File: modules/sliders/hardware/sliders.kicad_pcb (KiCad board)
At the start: 2 copper layers, 157.5 x 96.5 mm, 10 parts, among them J5 Button

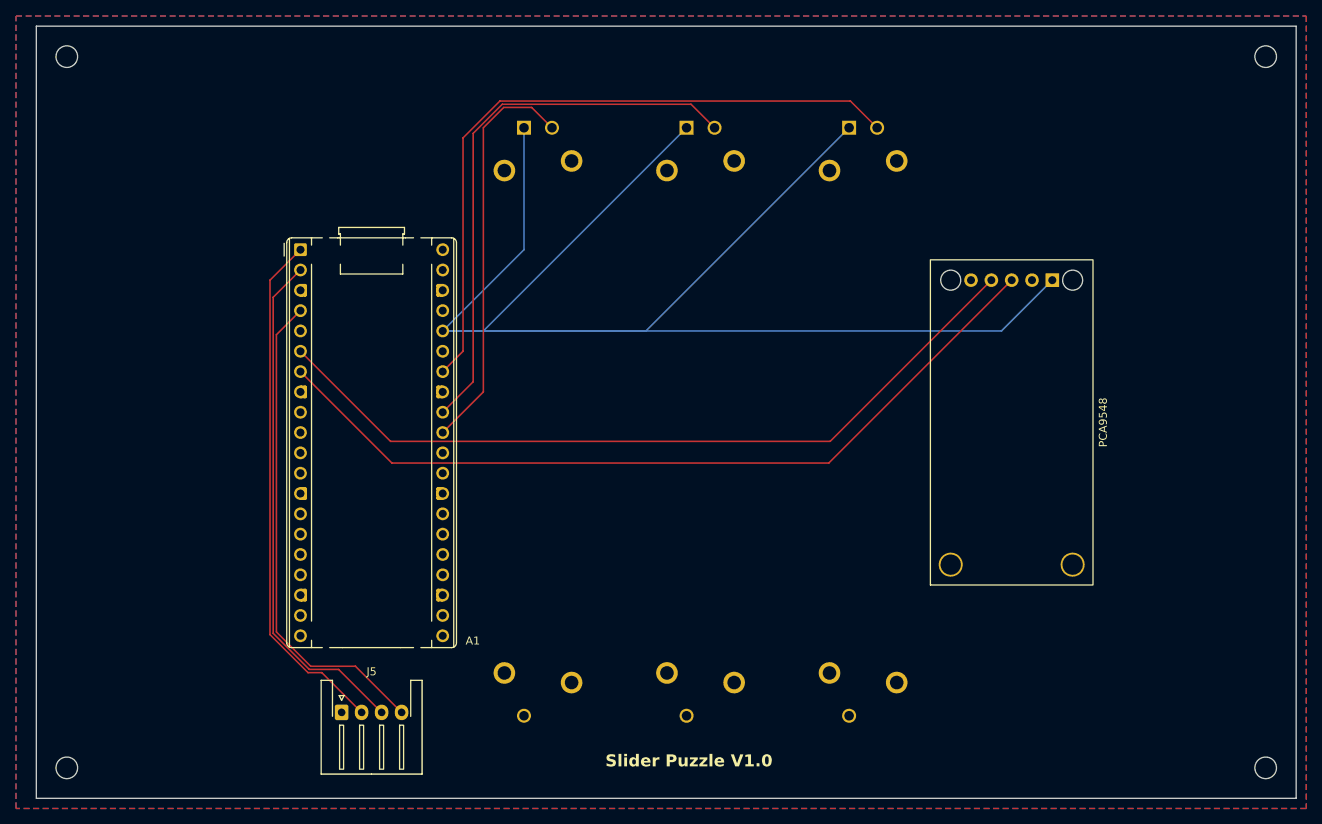
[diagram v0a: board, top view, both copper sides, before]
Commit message: Modified Slider PCB Design
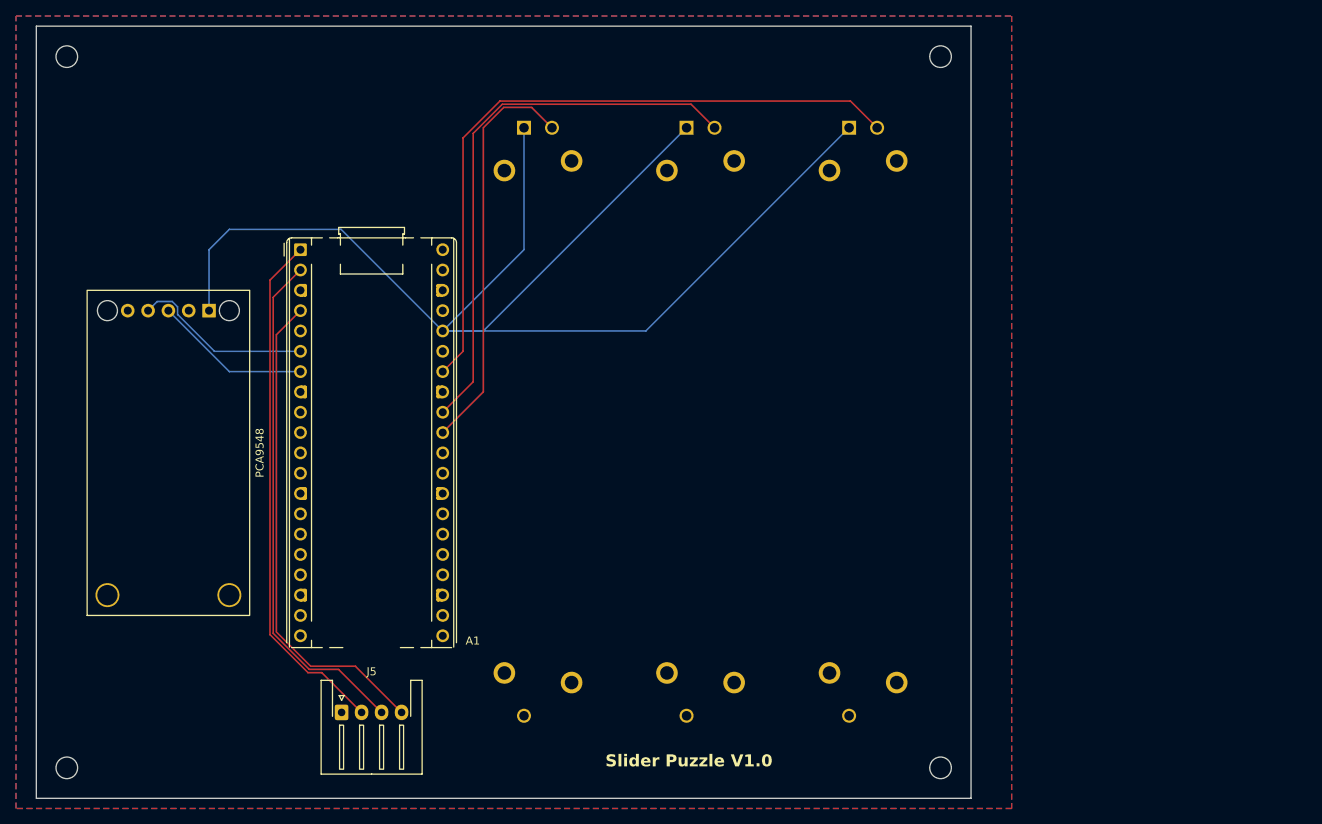
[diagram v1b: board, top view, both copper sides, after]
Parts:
- A1: footprint Module:RaspberryPi_Pico_Common_THT -> Module:RaspberryPi_Pico_Common_THT_no_antenna
- moved PCA9548 105.5 mm to (72.4, 91.4)
- moved REF** 40.6 mm to (168.9, 130.8)
- moved REF** 40.6 mm to (168.9, 41.9)
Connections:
- VR1 pad MP: GND -> (no net)
- VR2 pad MP: GND -> (no net)
- VR3 pad MP: GND -> (no net)
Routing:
- net /SCL_0: track 103.1 -> 19.7 mm
- net /SDA_0: track 99.4 -> 22.7 mm
- net /3.3v: track 210.8 -> 175.1 mm
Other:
- board size 157.5 x 96.5 mm -> 116.8 x 96.5 mm
